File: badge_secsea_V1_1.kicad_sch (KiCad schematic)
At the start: 132 parts, among them J1 USB_C_Receptacle_USB2.0_14P, J4 AFC07-S24ECA-00, J5 Micro_SD_Card_Det1, Q1 2N7002, Q2 SI1308EDL, Q3 SI2301, SW1 TS-1187A-B-A-B, SW2 K2-1112SW-A4SW-04, SW3 K2-1112SW-A4SW-04, SW4 XDTD-6650, SW5 XDTD-6650, SW6 TS-1187A-B-A-B, SW7 SW_SPDT, U1 RP2040, U2 74HC139, U3 W25Q128JVSIQ, U4 CC1101RGPR, U5 TP4056, U6 TPS63000, U7 LM321, X1 ABM8-272-T3, X2 26MHz

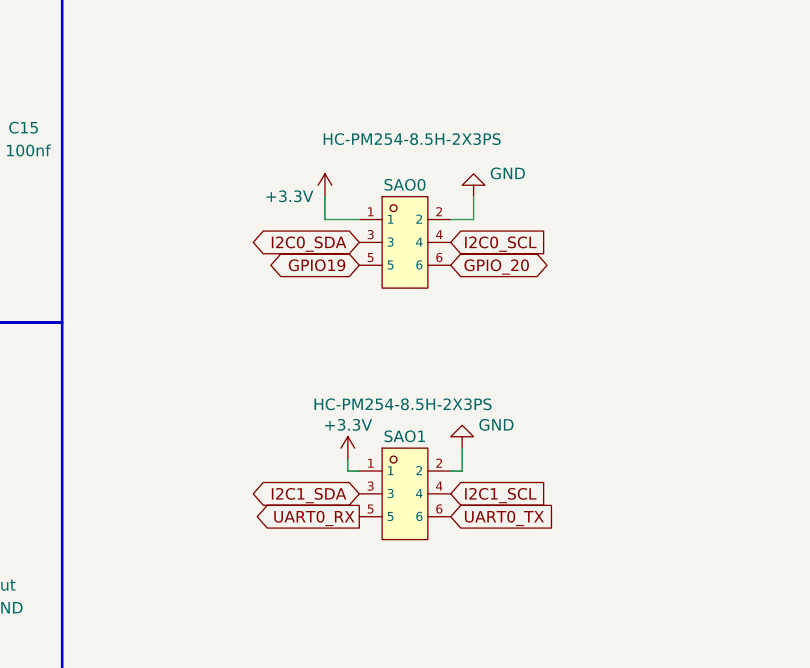
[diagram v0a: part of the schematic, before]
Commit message: Review with Miaou
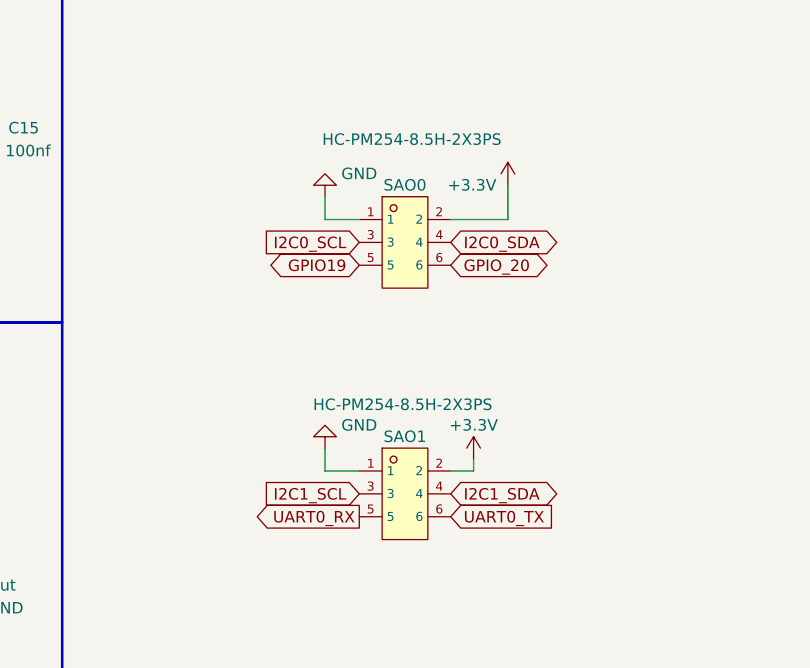
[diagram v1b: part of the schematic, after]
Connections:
- net +3.3V: now also SAO0.2, SAO1.2; no longer SAO0.1, SAO1.1
- net GND: now also SAO0.1, SAO1.1; no longer SAO0.2, SAO1.2
- net I2C0_SCL: now also SAO0.3; no longer SAO0.4
- net I2C0_SDA: now also SAO0.4; no longer SAO0.3
- net I2C1_SCL: now also SAO1.3; no longer SAO1.4
- net I2C1_SDA: now also SAO1.4; no longer SAO1.3
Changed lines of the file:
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@@
 	(wire
 		(pts
-			(xy 403.86 303.53) (xy 403.86 302.26)
+			(xy 316.23 186.69) (xy 316.23 189.23)
 		)
 		(stroke
@@
 	(wire
 		(pts
-			(xy 316.23 186.69) (xy 316.23 189.23)
+			(xy 204.47 256.54) (xy 215.9 256.54)
 		)
 		(stroke
@@
 	(wire
 		(pts
-			(xy 204.47 256.54) (xy 215.9 256.54)
+			(xy 228.6 71.12) (xy 229.87 71.12)
 		)
 		(stroke
@@
 	(wire
 		(pts
-			(xy 228.6 71.12) (xy 229.87 71.12)
+			(xy 421.64 275.59) (xy 421.64 271.78)
 		)
 		(stroke
@@
 	(wire
 		(pts
-			(xy 73.66 151.13) (xy 73.66 153.67)
+			(xy 417.83 303.53) (xy 417.83 302.26)
 		)
 		(stroke
@@
 	(wire
 		(pts
-			(xy 312.42 177.8) (xy 316.23 177.8)
+			(xy 73.66 151.13) (xy 73.66 153.67)
 		)
 		(stroke
@@
 	(wire
 		(pts
-			(xy 158.75 293.37) (xy 161.29 293.37)
+			(xy 312.42 177.8) (xy 316.23 177.8)
 		)
 		(stroke
@@
 	(wire
 		(pts
-			(xy 125.73 270.51) (xy 125.73 278.13)
+			(xy 158.75 293.37) (xy 161.29 293.37)
 		)
 		(stroke
@@
 	(wire
 		(pts
-			(xy 203.2 71.12) (xy 212.09 71.12)
+			(xy 125.73 270.51) (xy 125.73 278.13)
 		)
 		(stroke
@@
 	(wire
 		(pts
-			(xy 415.29 275.59) (xy 417.83 275.59)
+			(xy 203.2 71.12) (xy 212.09 71.12)
 		)
 		(stroke
@@
 	(wire
 		(pts
-			(xy 101.6 270.51) (xy 99.06 270.51)
+			(xy 401.32 300.99) (xy 401.32 303.53)
 		)
 		(stroke
@@
 	(wire
 		(pts
-			(xy 86.36 266.7) (xy 86.36 270.51)
+			(xy 101.6 270.51) (xy 99.06 270.51)
 		)
 		(stroke
@@
 	(wire
 		(pts
-			(xy 417.83 275.59) (xy 417.83 273.05)
+			(xy 86.36 266.7) (xy 86.36 270.51)
 		)
 		(stroke
@@
 	(wire
 		(pts
-			(xy 405.13 303.53) (xy 403.86 303.53)
-		)
-		(stroke
-			(width 0)
-			(type default)
-		)
-	)
-	(wire
-		(pts
 			(xy 106.68 78.74) (xy 101.6 78.74)
 		)
@@
 	(wire
 		(pts
-			(xy 416.56 303.53) (xy 415.29 303.53)
-		)
-		(stroke
-			(width 0)
-			(type default)
-		)
-	)
-	(wire
-		(pts
 			(xy 153.67 139.7) (xy 151.13 139.7)
 		)
@@
 	(wire
 		(pts
+			(xy 415.29 303.53) (xy 417.83 303.53)
+		)
+		(stroke
+			(width 0)
+			(type default)
+		)
+	)
+	(wire
+		(pts
 			(xy 78.74 158.75) (xy 78.74 153.67)
 		)
@@
 	(wire
 		(pts
-			(xy 405.13 275.59) (xy 401.32 275.59)
-		)
-		(stroke
-			(width 0)
-			(type default)
-		)
-	)
-	(wire
-		(pts
 			(xy 408.94 186.69) (xy 408.94 184.15)
 		)
@@
 	(wire
 		(pts
-			(xy 401.32 273.05) (xy 401.32 275.59)
-		)
-		(stroke
-			(width 0)
-			(type default)
-		)
-	)
-	(wire
-		(pts
 			(xy 355.6 177.8) (xy 355.6 181.61)
 		)
@@
 	(wire
 		(pts
-			(xy 416.56 300.99) (xy 416.56 303.53)
-		)
-		(stroke
-			(width 0)
-			(type default)
-		)
-	)
-	(wire
-		(pts
 			(xy 144.78 318.77) (xy 134.62 318.77)
 		)
@@
 	(wire
 		(pts
+			(xy 401.32 275.59) (xy 401.32 273.05)
+		)
+		(stroke
+			(width 0)
+			(type default)
+		)
+	)
+	(wire
+		(pts
 			(xy 72.39 173.99) (xy 78.74 173.99)
 		)
@@
 	(wire
 		(pts
+			(xy 401.32 303.53) (xy 405.13 303.53)
+		)
+		(stroke
+			(width 0)
+			(type default)
+		)
+	)
+	(wire
+		(pts
 			(xy 255.27 73.66) (xy 265.43 73.66)
 		)
@@
 	(wire
 		(pts
+			(xy 415.29 275.59) (xy 421.64 275.59)
+		)
+		(stroke
+			(width 0)
+			(type default)
+		)
+	)
+	(wire
+		(pts
 			(xy 407.67 213.36) (xy 405.13 213.36)
 		)
@@
 	(wire
 		(pts
+			(xy 405.13 275.59) (xy 401.32 275.59)
+		)
+		(stroke
+			(width 0)
+			(type default)
+		)
+	)
+	(wire
+		(pts
 			(xy 82.55 163.83) (xy 82.55 168.91)
 		)
@@
 	(global_label "I2C0_SDA"
 		(shape bidirectional)
-		(at 405.13 278.13 180)
+		(at 415.29 278.13 0)
 		(effects
 			(font
 				(size 1.27 1.27)
 			)
-			(justify right)
+			(justify left)
 		)
 		(property "Intersheetrefs" "${INTERSHEET_REFS}"
-			(at 405.13 278.13 0)
+			(at 415.29 278.13 0)
 			(hide yes)
 			(show_name no)
@@
 	(global_label "I2C1_SCL"
 		(shape input)
-		(at 415.29 306.07 0)
+		(at 405.13 306.07 180)
 		(effects
 			(font
 				(size 1.27 1.27)
 			)
-			(justify left)
+			(justify right)
 		)
 		(property "Intersheetrefs" "${INTERSHEET_REFS}"
-			(at 415.29 306.07 0)
+			(at 405.13 306.07 0)
 			(hide yes)
 			(show_name no)
@@
 	(global_label "I2C1_SDA"
 		(shape bidirectional)
-		(at 405.13 306.07 180)
+		(at 415.29 306.07 0)
 		(effects
 			(font
 				(size 1.27 1.27)
 			)
-			(justify right)
+			(justify left)
 		)
 		(property "Intersheetrefs" "${INTERSHEET_REFS}"
-			(at 405.13 306.07 0)
+			(at 415.29 306.07 0)
 			(hide yes)
 			(show_name no)
@@
 	(global_label "I2C0_SCL"
 		(shape input)
-		(at 415.29 278.13 0)
+		(at 405.13 278.13 180)
 		(effects
 			(font
 				(size 1.27 1.27)
 			)
-			(justify left)
+			(justify right)
 		)
 		(property "Intersheetrefs" "${INTERSHEET_REFS}"
-			(at 415.29 278.13 0)
+			(at 405.13 278.13 0)
 			(hide yes)
 			(show_name no)
@@
 	(symbol
 		(lib_id "power:+3.3V")
-		(at 403.86 302.26 0)
+		(at 417.83 302.26 0)
 		(unit 1)
 		(body_style 1)
@@
 		(dnp no)
 		(property "Reference" "#PWR058"
-			(at 403.86 306.07 0)
+			(at 417.83 306.07 0)
 			(hide yes)
 			(show_name no)
@@
 		)
 		(property "Value" "+3.3V"
-			(at 403.86 298.45 0)
+			(at 417.83 298.45 0)
 			(show_name no)
 			(do_not_autoplace no)
@@
 		)
 		(property "Footprint" ""
-			(at 403.86 302.26 0)
+			(at 417.83 302.26 0)
 			(hide yes)
 			(show_name no)
@@
 		)
 		(property "Datasheet" ""
-			(at 403.86 302.26 0)
+			(at 417.83 302.26 0)
 			(hide yes)
 			(show_name no)
@@
 		)
 		(property "Description" "Power symbol creates a global label with name \"+3.3V\""
-			(at 403.86 302.26 0)
+			(at 417.83 302.26 0)
 			(hide yes)
 			(show_name no)
@@
 	(symbol
 		(lib_id "power:GND")
-		(at 416.56 300.99 180)
+		(at 401.32 300.99 180)
 		(unit 1)
 		(body_style 1)
@@
 		(dnp no)
 		(property "Reference" "#PWR013"
-			(at 416.56 294.64 0)
+			(at 401.32 294.64 0)
 			(hide yes)
 			(show_name no)
@@
 		)
 		(property "Value" "GND"
-			(at 420.37 298.45 0)
+			(at 405.13 298.45 0)
 			(show_name no)
 			(do_not_autoplace no)
@@
 		)
 		(property "Footprint" ""
-			(at 416.56 300.99 0)
+			(at 401.32 300.99 0)
 			(hide yes)
 			(show_name no)
@@
 		)
 		(property "Datasheet" ""
-			(at 416.56 300.99 0)
+			(at 401.32 300.99 0)
 			(hide yes)
 			(show_name no)
@@
 		)
 		(property "Description" "Power symbol creates a global label with name \"GND\" , ground"
-			(at 416.56 300.99 0)
+			(at 401.32 300.99 0)
 			(hide yes)
 			(show_name no)
@@
 	(symbol
 		(lib_id "power:GND")
-		(at 417.83 273.05 180)
+		(at 401.32 273.05 180)
 		(unit 1)
 		(body_style 1)
@@
 		(dnp no)
 		(property "Reference" "#PWR067"
-			(at 417.83 266.7 0)
+			(at 401.32 266.7 0)
 			(hide yes)
 			(show_name no)
@@
 		)
 		(property "Value" "GND"
-			(at 421.64 270.51 0)
+			(at 405.13 270.51 0)
 			(show_name no)
 			(do_not_autoplace no)
@@
 		)
 		(property "Footprint" ""
-			(at 417.83 273.05 0)
+			(at 401.32 273.05 0)
 			(hide yes)
 			(show_name no)
@@
 		)
 		(property "Datasheet" ""
-			(at 417.83 273.05 0)
+			(at 401.32 273.05 0)
 			(hide yes)
 			(show_name no)
@@
 		)
 		(property "Description" "Power symbol creates a global label with name \"GND\" , ground"
-			(at 417.83 273.05 0)
+			(at 401.32 273.05 0)
 			(hide yes)
 			(show_name no)
@@
 	(symbol
 		(lib_id "power:+3.3V")
-		(at 401.32 273.05 0)
+		(at 421.64 271.78 0)
 		(unit 1)
 		(body_style 1)
@@
 		(dnp no)
 		(property "Reference" "#PWR066"
-			(at 401.32 276.86 0)
+			(at 421.64 275.59 0)
 			(hide yes)
 			(show_name no)
@@
 		)
 		(property "Value" "+3.3V"
-			(at 400.05 273.05 0)
+			(at 420.37 271.78 0)
 			(show_name no)
 			(do_not_autoplace yes)
@@
 		)
 		(property "Footprint" ""
-			(at 401.32 273.05 0)
+			(at 421.64 271.78 0)
 			(hide yes)
 			(show_name no)
@@
 		)
 		(property "Datasheet" ""
-			(at 401.32 273.05 0)
+			(at 421.64 271.78 0)
 			(hide yes)
 			(show_name no)
@@
 		)
 		(property "Description" "Power symbol creates a global label with name \"+3.3V\""
-			(at 401.32 273.05 0)
+			(at 421.64 271.78 0)
 			(hide yes)
 			(show_name no)
